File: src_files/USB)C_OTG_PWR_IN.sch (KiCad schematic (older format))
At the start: 51 parts, among them U13 STWLC68, U14 TPS56637RPAR

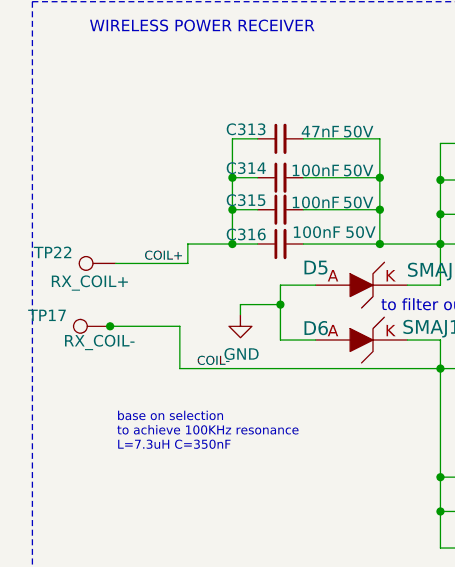
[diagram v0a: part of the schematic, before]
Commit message: layout change
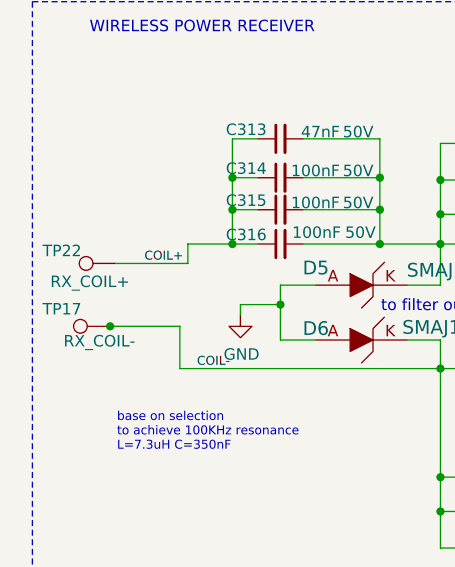
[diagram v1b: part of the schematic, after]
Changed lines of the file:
@@
 AR Path="/626A6204/62FDE5CD" Ref="TP?"  Part="1"
 AR Path="/6823D52E/62FDE5CD" Ref="TP22"  Part="1"
-F 0 "TP22" V 869 1858 50  0000 L CNN
+F 0 "TP22" V 860 1820 50  0000 L CNN
 F 1 "RX_COIL+" V 995 1610 50  0000 L CNN
 F 2 "TestPoint:TestPoint_Pad_1.5x1.5mm" H 1115 1670 50  0001 C CNN
@@
 AR Path="/626A6204/62FDE5D4" Ref="TP?"  Part="1"
 AR Path="/6823D52E/62FDE5D4" Ref="TP17"  Part="1"
-F 0 "TP17" V 844 2133 50  0000 L CNN
+F 0 "TP17" V 815 2070 50  0000 L CNN
 F 1 "RX_COIL-" V 955 1835 50  0000 L CNN
 F 2 "TestPoint:TestPoint_Pad_1.5x1.5mm" H 1090 1945 50  0001 C CNN
